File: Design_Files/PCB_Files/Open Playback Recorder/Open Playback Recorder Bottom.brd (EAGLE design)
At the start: 100 x 50 mm, 17 parts, among them J2 SJ1-3535NG, J3 SJ1-3535NG

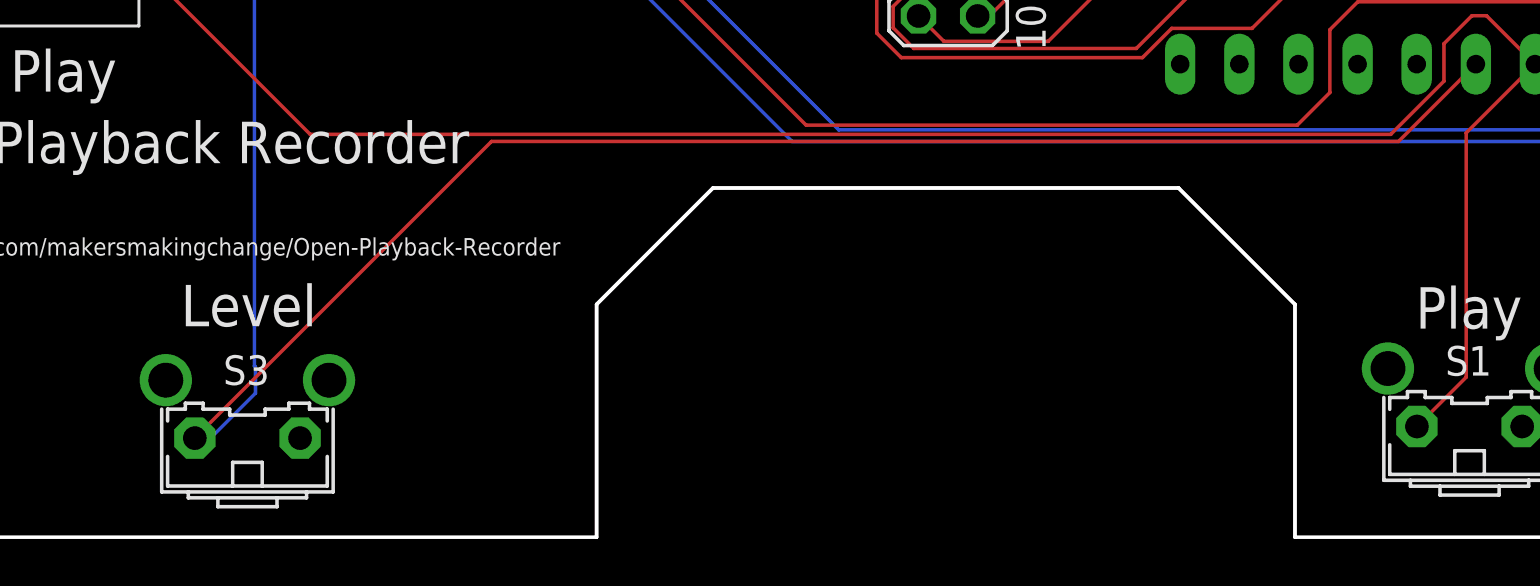
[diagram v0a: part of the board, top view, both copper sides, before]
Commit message: Minor changes to build files
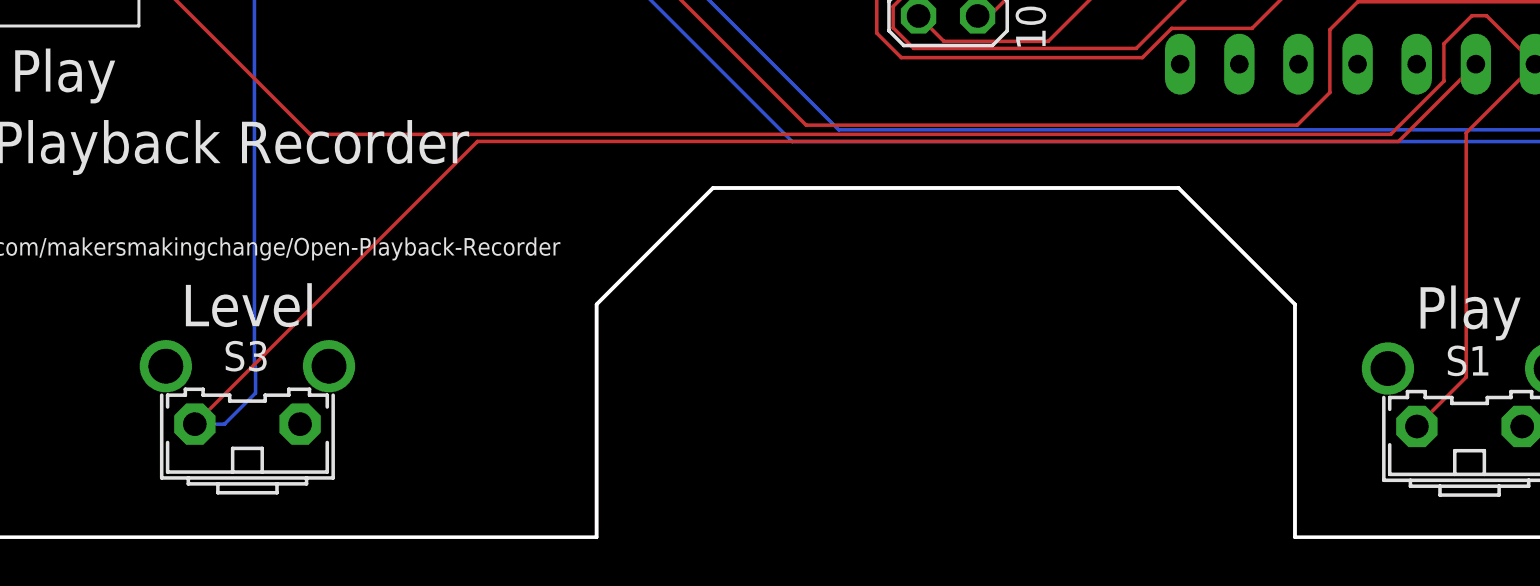
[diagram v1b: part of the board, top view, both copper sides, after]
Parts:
- moved S3 0.60 mm to (20.0, 6.10)
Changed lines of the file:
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@@
 </layers>
 <board>
-<fusionsync huburn="a.YnVzaW5lc3M6bmVpbHNxdWlyZQ" projecturn="a.YnVzaW5lc3M6bmVpbHNxdWlyZSMyMDIyMTIxMjU4ODQ4MDM4MQ" f3durn="urn:adsk.wipprod:dm.lineage:RpvBgM7aRKqYAMB9V_E1Dw" pcbguid="" lastpulledtime="2024-05-27T18:29:35Z" lastsyncedchangeguid="" latestrevisionid="6d18fd68-a1bb-43dc-acf0-3cef81a52a5e" lastsyncedrevisionid="6d18fd68-a1bb-43dc-acf0-3cef81a52a5e" lastboardhashguid="7ff0344c-72ac-49de-0f7e-615c607258a4" lastpushedtime="2024-06-17T17:31:42Z" linktopcb3d="true"/>
+<fusionsync huburn="a.YnVzaW5lc3M6bmVpbHNxdWlyZQ" projecturn="a.YnVzaW5lc3M6bmVpbHNxdWlyZSMyMDIyMTIxMjU4ODQ4MDM4MQ" f3durn="urn:adsk.wipprod:dm.lineage:RpvBgM7aRKqYAMB9V_E1Dw" pcbguid="" lastpulledtime="2024-05-27T18:29:35Z" lastsyncedchangeguid="" latestrevisionid="6d18fd68-a1bb-43dc-acf0-3cef81a52a5e" lastsyncedrevisionid="6d18fd68-a1bb-43dc-acf0-3cef81a52a5e" lastboardhashguid="7ff0344c-72ac-49de-0f7e-615c607258a4" lastpushedtime="2024-06-17T17:31:42Z" linktopcb3d="false"/>
 <plain>
 <text x="9.31" y="36.95" size="1.778" layer="25">Level</text>
@@
 <attribute name="VALUE" x="81.317" y="0.031" size="1.27" layer="27" ratio="10"/>
 </element>
-<element name="S3" library="MMC_Eagle" library_urn="urn:adsk.eagle:library:44377252" package="B3F-31XX" package3d_urn="urn:adsk.eagle:package:44377697/1" value="" x="20" y="5.5" smashed="yes">
-<attribute name="NAME" x="18.96" y="6.54" size="1.27" layer="25" ratio="10"/>
-<attribute name="VALUE" x="16.317" y="-0.469" size="1.27" layer="27" ratio="10"/>
+<element name="S3" library="MMC_Eagle" library_urn="urn:adsk.eagle:library:44377252" package="B3F-31XX" package3d_urn="urn:adsk.eagle:package:44377697/1" value="" x="20" y="6.1" smashed="yes">
+<attribute name="NAME" x="18.96" y="7.14" size="1.27" layer="25" ratio="10"/>
+<attribute name="VALUE" x="16.317" y="0.131" size="1.27" layer="27" ratio="10"/>
 </element>
 <element name="U$6" library="MMC_Eagle" library_urn="urn:adsk.eagle:library:44377252" package="SWITCH_SPDT_11MA1QS1" package3d_urn="urn:adsk.eagle:package:44377752/1" value="SWITCH-SPDT-OS102011" x="96.5" y="43.5" smashed="yes" rot="R90"/>
@@
 <contactref element="U$1" pad="D3"/>
 <contactref element="S3" pad="1"/>
-<wire x1="17.7394" y1="4.2554" x2="30.484" y2="17" width="0.1524" layer="1"/>
+<wire x1="17.7394" y1="4.8554" x2="29.884" y2="17" width="0.1524" layer="1"/>
 <wire x1="69.45" y1="17" x2="72.77" y2="20.32" width="0.1524" layer="1"/>
-<wire x1="30.484" y1="17" x2="69.45" y2="17" width="0.1524" layer="1"/>
+<wire x1="29.884" y1="17" x2="69.45" y2="17" width="0.1524" layer="1"/>
 <wire x1="6.9574" y1="42.30899375" x2="7.93299375" y2="41.3334" width="0.1524" layer="16"/>
 <wire x1="7.93299375" y1="41.3334" x2="9.84700625" y2="41.3334" width="0.1524" layer="16"/>
@@
 <wire x1="4.94" y1="45.37" x2="6.9574" y2="43.3526" width="0.1524" layer="16"/>
 <wire x1="9.84700625" y1="41.3334" x2="11.88360625" y2="43.37" width="0.1524" layer="16"/>
-<wire x1="17.7394" y1="4.2554" x2="18.4184" y2="4.2554" width="0.1524" layer="16"/>
-<wire x1="18.4184" y1="4.2554" x2="20.34735" y2="6.18435" width="0.1524" layer="16"/>
+<wire x1="17.7394" y1="4.8554" x2="19.0184" y2="4.8554" width="0.1524" layer="16"/>
+<wire x1="19.0184" y1="4.8554" x2="20.34735" y2="6.18435" width="0.1524" layer="16"/>
 <wire x1="20.34735" y1="6.18435" x2="20.34735" y2="7.30485" width="0.1524" layer="16"/>
 <wire x1="20.34735" y1="7.30485" x2="20.3" y2="7.3522" width="0.1524" layer="16"/>
